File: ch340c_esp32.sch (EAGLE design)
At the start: 13 parts, among them J1 CQ-USB-C16PSMT01, U1 AMS1117 3.3V, U2 CH340C, U3 AO3400, U4 AO3400

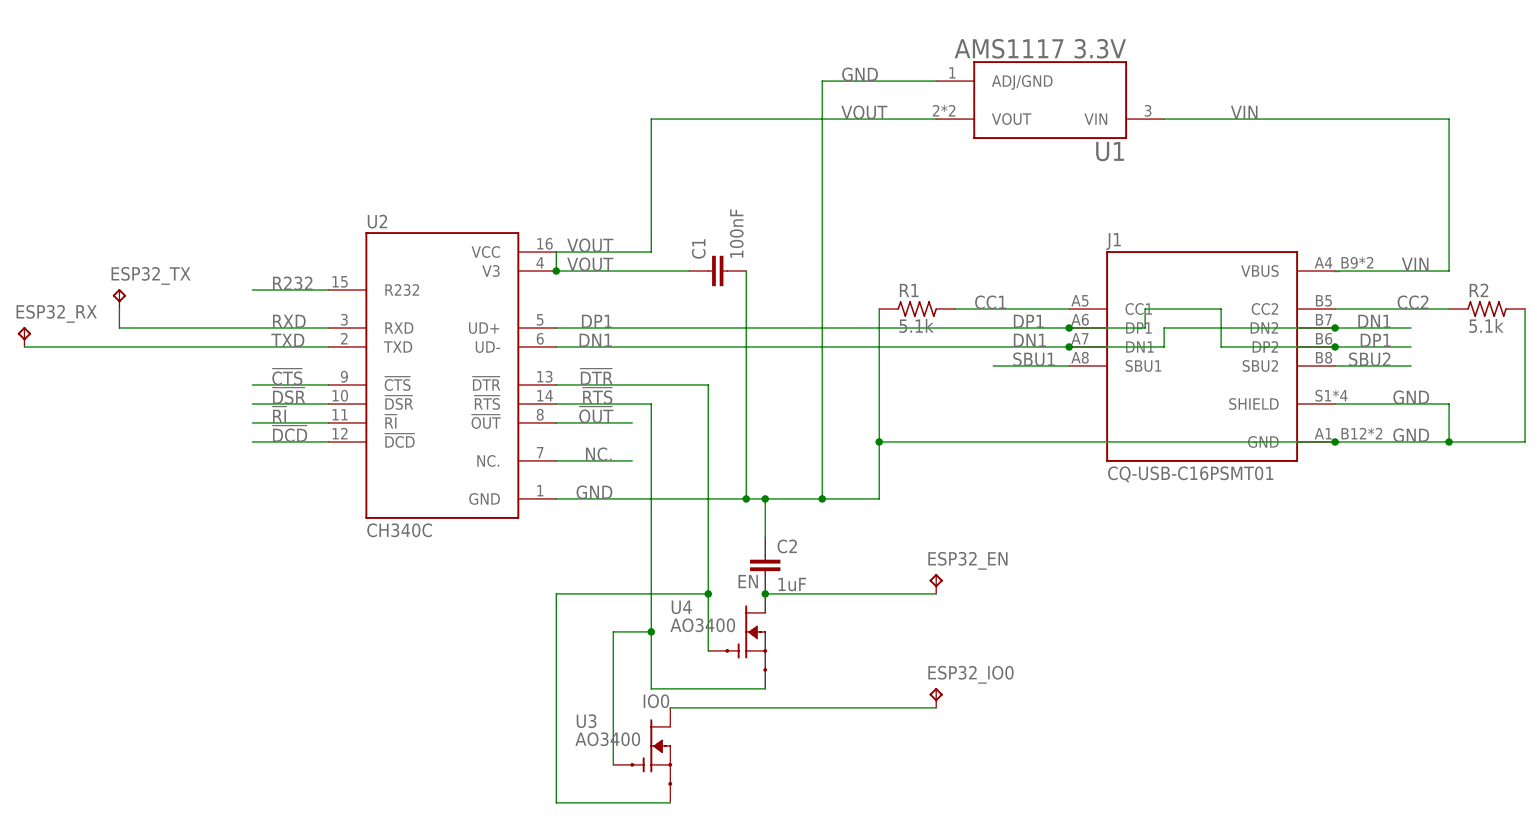
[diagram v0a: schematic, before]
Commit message: prototype v1.1
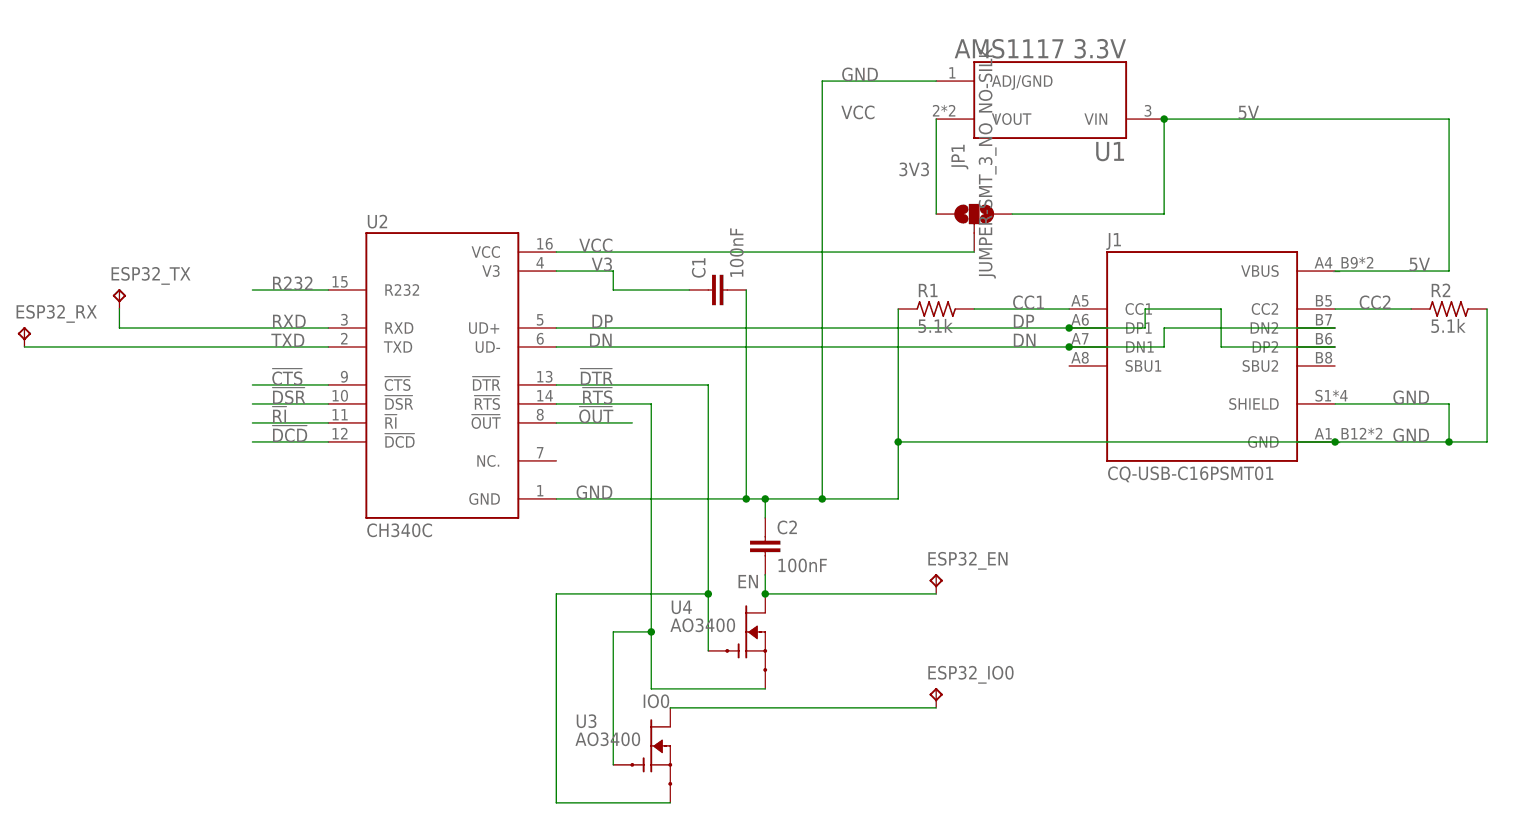
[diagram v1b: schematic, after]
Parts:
- added JP1: JUMPER-SMT_3_NO_NO-SILK, SparkFun-Jumpers:JUMPER-SMT_3_NO_NO-SILK
- C2: value 1uF -> 100nF
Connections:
- net DN1 renamed DN
- net DP1 renamed DP
- removed net NC.: U2.NC.
- removed net SBU1: J1.SBU1
- removed net SBU2: J1.SBU2
- removed net VIN: J1.VBUS, U1.VIN
- removed net VOUT: C1.1, U1.VOUT, U2.V3, U2.VCC
- new net 3V3: JP1.1, U1.VOUT
- new net 5V: J1.VBUS, JP1.3, U1.VIN
- new net V3: C1.1, U2.V3
- new net VCC: JP1.2, U2.VCC
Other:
- moved on the sheet: C1, C2, R1, R2
